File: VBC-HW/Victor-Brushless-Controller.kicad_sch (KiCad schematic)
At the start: 81 parts, among them J1 i2c/UART, P1 V+, P2 GND, Q1 TPH4R008NH, Q2 TPH4R008NH, Q3 TPH4R008NH, Q4 TPH4R008NH, Q5 TPH4R008NH, Q6 TPH4R008NH, SW1 BOOT, SW2 RESET, U1 DRV8305NQPHPRQ1, U2 ESP-WROOM-32E, U3 LMR14010ADDCR, U5 STLM20W87F, U6 SPI, U7 AS5047P-ATSM_C962063

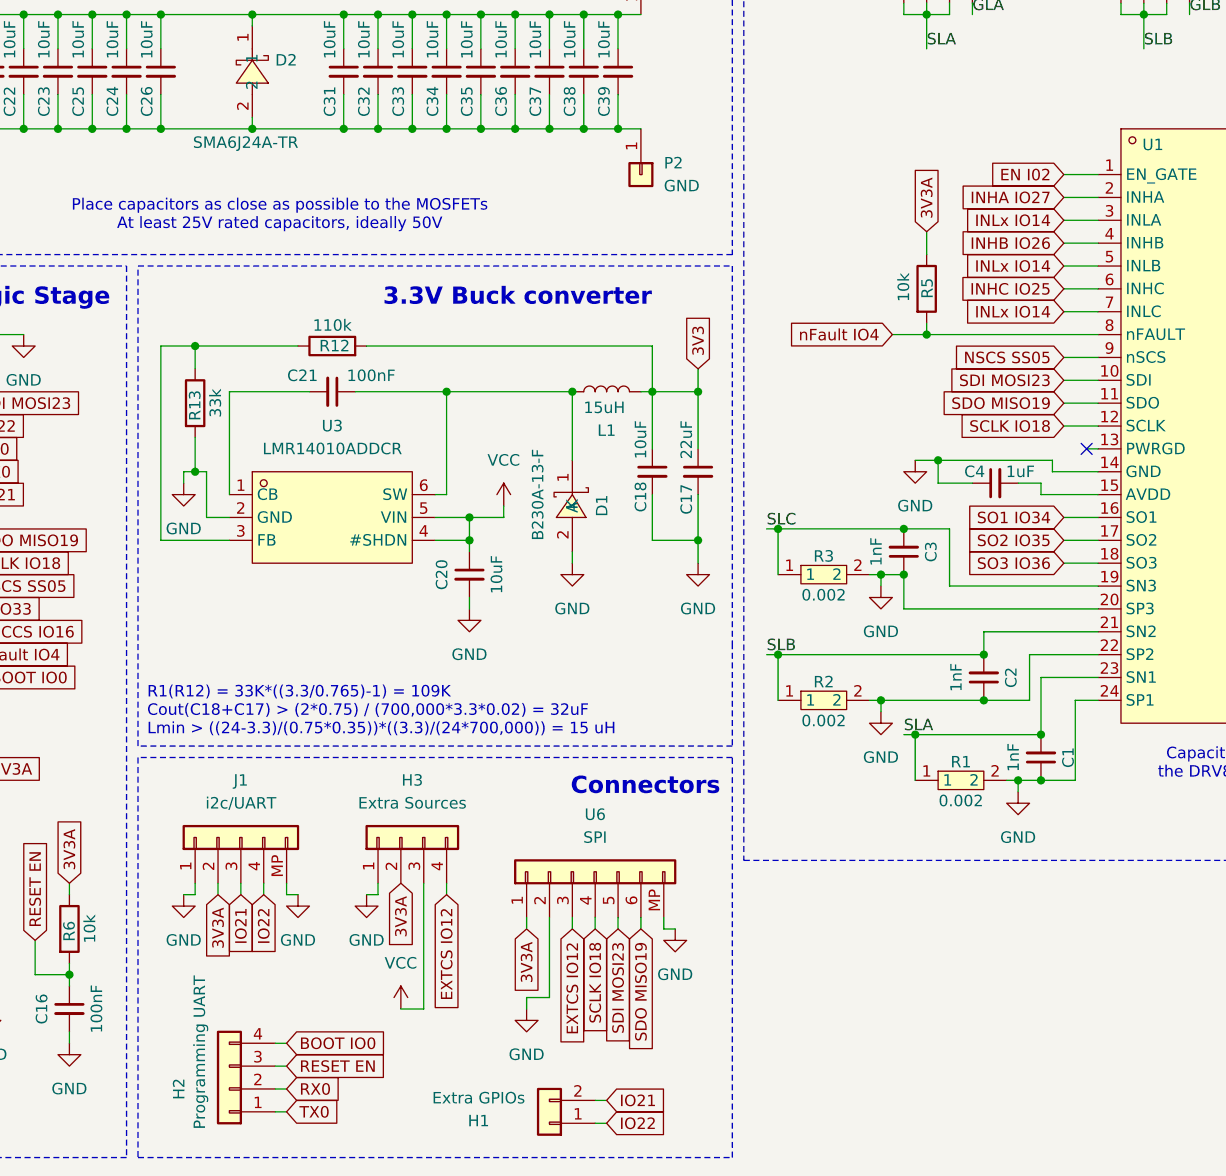
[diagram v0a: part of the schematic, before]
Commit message: Finished all connections
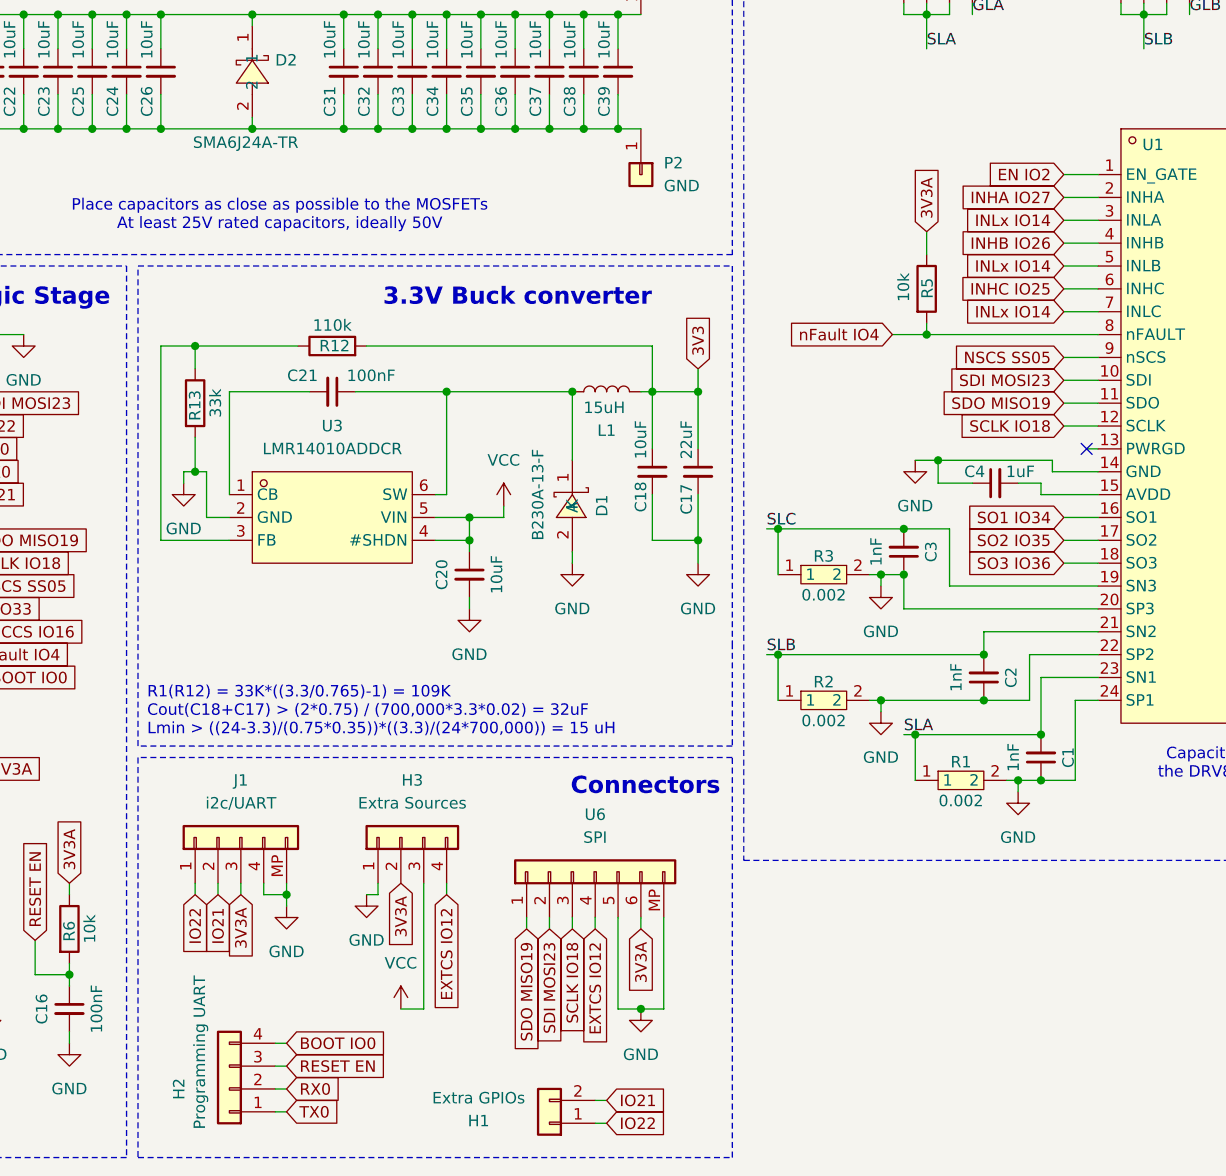
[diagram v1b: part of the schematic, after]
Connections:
- net EN I02 is gone; now on net EN IO2: U1.1 (EN_GATE)
- net 3V3A: now also J1.3 (Pin_3), U6.6 (Pin_6); no longer J1.2 (Pin_2), U6.1 (Pin_1)
- net EXTCS IO12: now also U6.4 (Pin_4); no longer U6.3 (Pin_3)
- net GND: now also J1.4 (Pin_4), U6.5 (Pin_5); no longer J1.1 (Pin_1), U6.2 (Pin_2)
- net IO21: now also J1.2 (Pin_2); no longer J1.3 (Pin_3)
- net IO22: now also J1.1 (Pin_1); no longer J1.4 (Pin_4)
- net SCLK IO18: now also U6.3 (Pin_3); no longer U6.4 (Pin_4)
- net SDI MOSI23: now also U6.2 (Pin_2); no longer U6.5 (Pin_5)
- net SDO MISO19: now also U6.1 (Pin_1); no longer U6.6 (Pin_6)
